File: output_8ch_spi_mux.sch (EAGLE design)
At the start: 52 parts, among them IC1 TPS706-1V8, IC2 5M160ZE64, IC3 SN75174SOIC-20, IC4 SN75174SOIC-20, IC6 STM32F042F, IC7 CAT24C256, Q1 50MHz

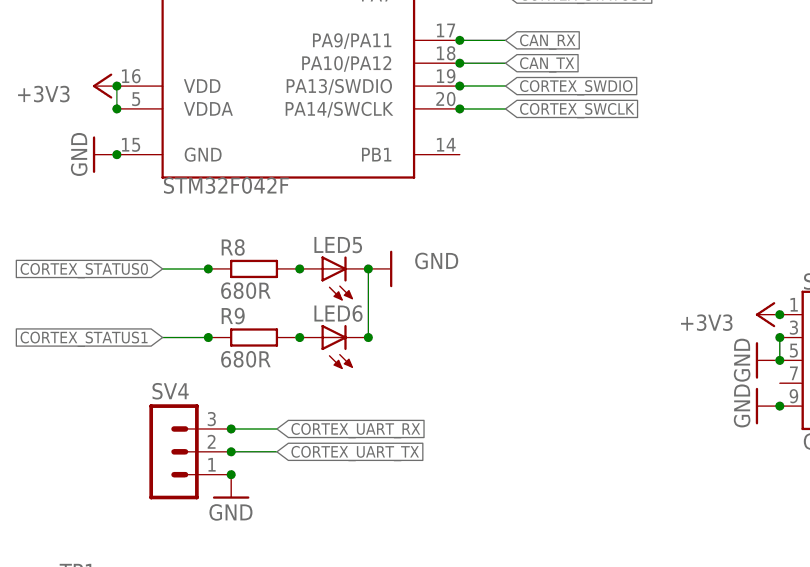
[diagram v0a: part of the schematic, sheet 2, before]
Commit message: yes
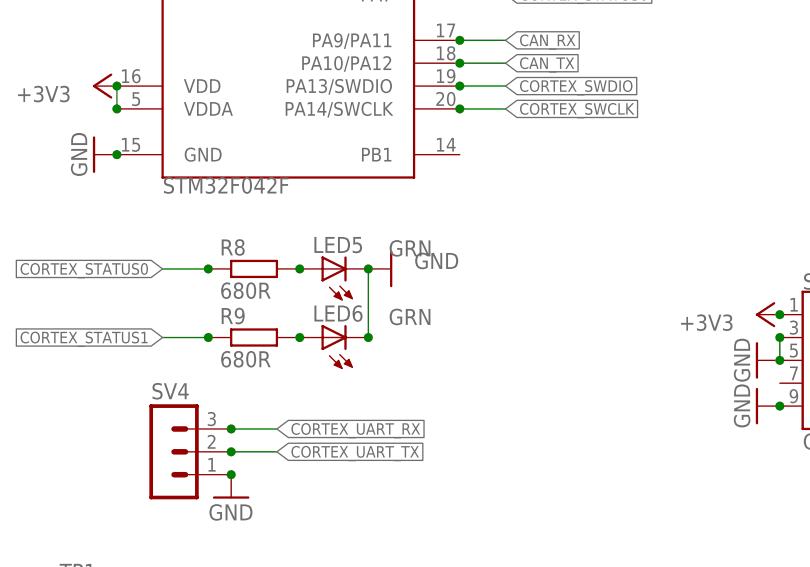
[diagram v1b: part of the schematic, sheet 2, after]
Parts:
- LED5, LED6: value (none) -> GRN
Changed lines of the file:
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@@
 <part name="GND6" library="supply1" library_urn="urn:adsk.eagle:library:371" deviceset="GND" device=""/>
 <part name="+3V33" library="supply1" library_urn="urn:adsk.eagle:library:371" deviceset="+3V3" device=""/>
-<part name="IC5" library="lichtenstein_onion" deviceset="TXB0108" device="TSSOP20"/>
+<part name="IC5" library="lichtenstein_onion" deviceset="TXB0108" device="TSSOP20" package3d_urn="urn:adsk.eagle:package:4349/2"/>
 <part name="+3V38" library="supply1" library_urn="urn:adsk.eagle:library:371" deviceset="+3V3" device=""/>
 <part name="GND17" library="supply1" library_urn="urn:adsk.eagle:library:371" deviceset="GND" device=""/>
@@
 </part>
 <part name="GND15" library="supply1" library_urn="urn:adsk.eagle:library:371" deviceset="GND" device=""/>
-<part name="IC1" library="lichtenstein_onion" deviceset="TPS706" device="SOT23-5" value="TPS706-1V8"/>
+<part name="IC1" library="lichtenstein_onion" deviceset="TPS706" device="SOT23-5" package3d_urn="urn:adsk.eagle:package:16456/2" value="TPS706-1V8"/>
 <part name="+3V32" library="supply1" library_urn="urn:adsk.eagle:library:371" deviceset="+3V3" device=""/>
 <part name="GND7" library="supply1" library_urn="urn:adsk.eagle:library:371" deviceset="GND" device=""/>
@@
 <attribute name="MOUSER" value="710-885012207072"/>
 </part>
-<part name="IC6" library="lichtenstein_onion" deviceset="STM32F042F" device=""/>
-<part name="LED5" library="led" library_urn="urn:adsk.eagle:library:259" deviceset="LED" device="CHIPLED_1206" package3d_urn="urn:adsk.eagle:package:15823/2">
+<part name="IC6" library="lichtenstein_onion" deviceset="STM32F042F" device="" package3d_urn="urn:adsk.eagle:package:4349/2"/>
+<part name="LED5" library="led" library_urn="urn:adsk.eagle:library:259" deviceset="LED" device="CHIPLED_1206" package3d_urn="urn:adsk.eagle:package:15823/2" value="GRN">
 <attribute name="MOUSER" value="604-APTR3216SGC"/>
 </part>
@@
 <attribute name="MOUSER" value="652-CR0805-FX6800GLF"/>
 </part>
-<part name="LED6" library="led" library_urn="urn:adsk.eagle:library:259" deviceset="LED" device="CHIPLED_1206" package3d_urn="urn:adsk.eagle:package:15823/2">
+<part name="LED6" library="led" library_urn="urn:adsk.eagle:library:259" deviceset="LED" device="CHIPLED_1206" package3d_urn="urn:adsk.eagle:package:15823/2" value="GRN">
 <attribute name="MOUSER" value="604-APTR3216SGC"/>
 </part>
@@
 <attribute name="MOUSER" x="139.7" y="83.82" size="1.27" layer="96" rot="R90" align="top-center" display="off"/>
 <attribute name="NAME" x="144.272" y="87.376" size="1.778" layer="95" rot="R180"/>
-<attribute name="VALUE" x="144.272" y="89.535" size="1.778" layer="96" rot="R180"/>
+<attribute name="VALUE" x="151.892" y="86.995" size="1.778" layer="96" rot="R180"/>
 </instance>
 <instance part="R8" gate="G$1" x="132.08" y="83.82" smashed="yes">
@@
 <attribute name="MOUSER" x="139.7" y="76.2" size="1.27" layer="96" rot="R90" align="top-center" display="off"/>
 <attribute name="NAME" x="144.272" y="79.756" size="1.778" layer="95" rot="R180"/>
-<attribute name="VALUE" x="144.272" y="81.915" size="1.778" layer="96" rot="R180"/>
+<attribute name="VALUE" x="151.892" y="79.375" size="1.778" layer="96" rot="R180"/>
 </instance>
 <instance part="GND35" gate="1" x="114.3" y="127" smashed="yes" rot="R270">
